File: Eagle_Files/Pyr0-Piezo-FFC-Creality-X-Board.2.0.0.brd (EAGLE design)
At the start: 8 parts, among them J1 FFC_MOLEX_0.5MM, J2 FFC_MOLEX_0.5MM

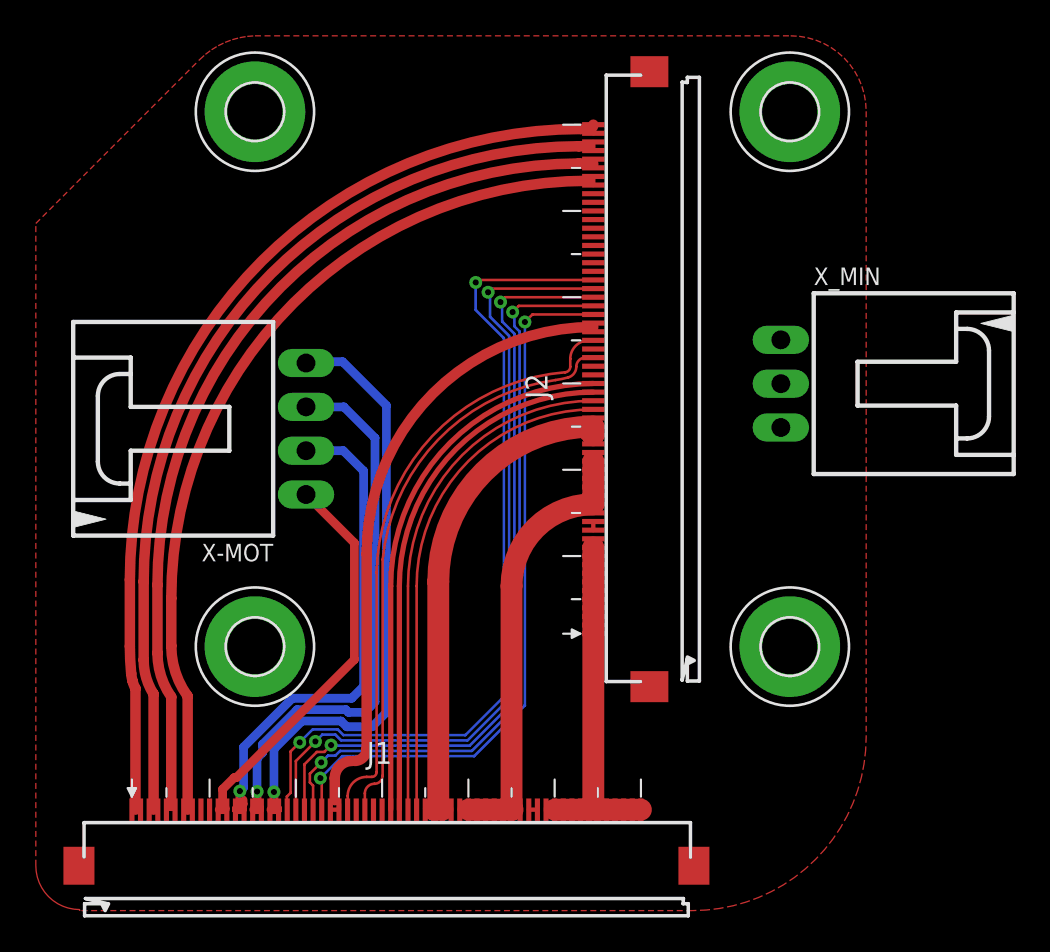
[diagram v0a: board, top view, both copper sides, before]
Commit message: Finished first iteration of x-gantry board
First version to address https://github.com/pyr0ball/pyr0piezo/issues/18
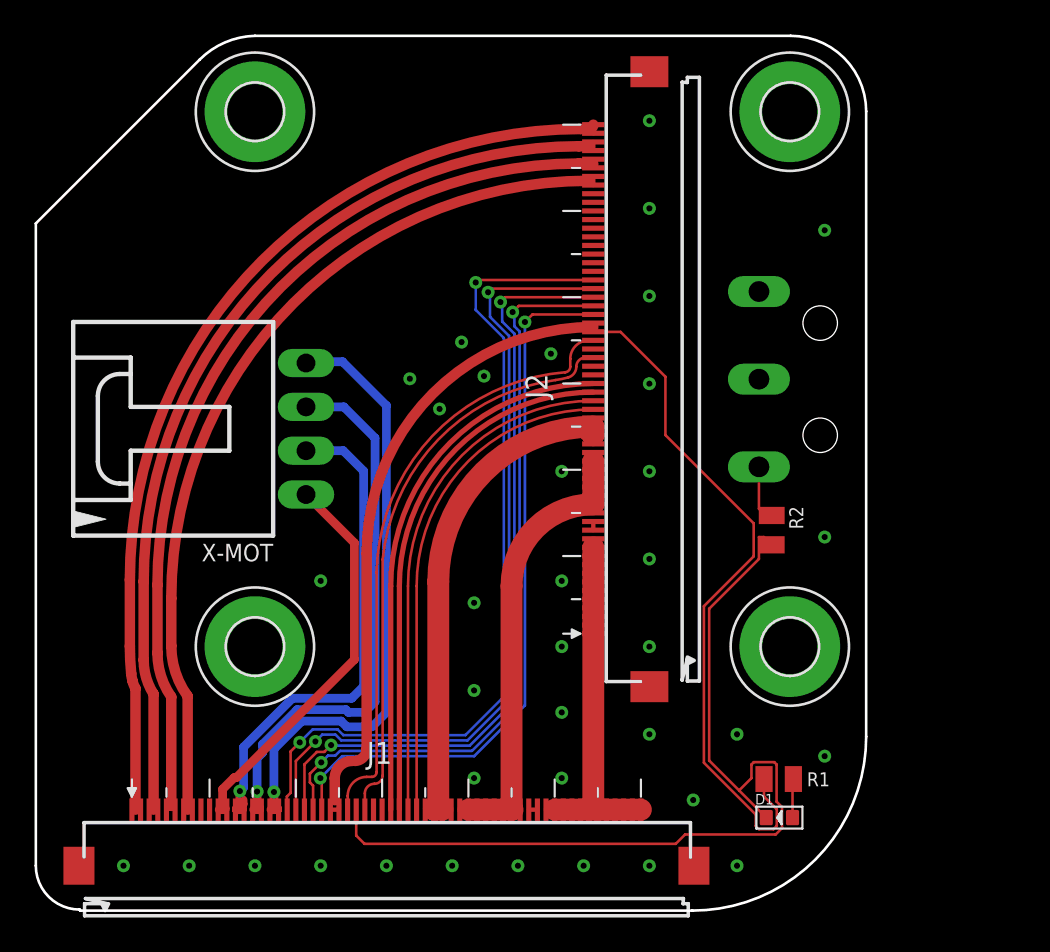
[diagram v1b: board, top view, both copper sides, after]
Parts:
- added D1: (no value), PiezoFFC:SEEED-LED_LED-0603
- added R1, R2: 1K, PiezoFFC:R0805
- X_MIN: value C-GRID-03-70553 -> LIMIT_SWITCHMICRO_SPDT_5.08; device PiezoFFC:70553-03 -> PiezoFFC:MICROSWITCH_5.08
- moved X_MIN 8.89 mm to (29.2, 15.5), flipped to the bottom, turned to 180 degrees
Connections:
- new net X_MIN_LED: D1.+, R1.1
- new net X_PULLDOWN: R2.1, X_MIN.P$1
- net AGND: now also X_MIN.P$2
- net VCC_REG: now also R1.2
- net X_MIN_TRIG: now also D1.-, R2.2
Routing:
- net X_MIN_TRIG: track 0.00 -> 53.7 mm
- net VCC_REG: track 35.4 -> 75.6 mm
- net X_PULLDOWN: track 0.00 -> 3.33 mm
- net X_MIN_LED: track 0.00 -> 2.25 mm
- net AGND: vias 0 -> 37
- added copper zone on layer 16, net AGND
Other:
- board outline added: 48.1 x 50.7 mm
